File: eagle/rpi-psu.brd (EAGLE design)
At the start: 50.8 x 50.8 mm, 19 parts, among them IC1 LD117AV33, IC2 TINY85P, Q1 TIP125, T1 2N2222

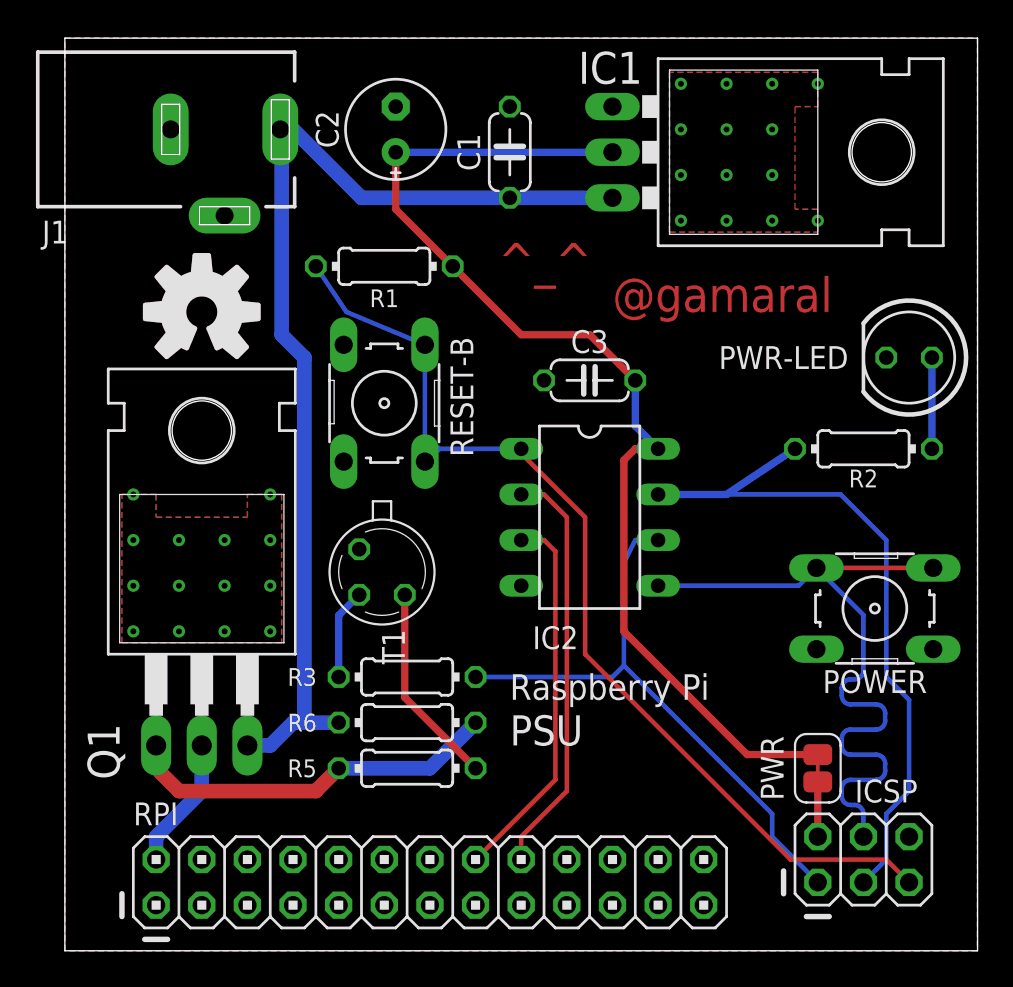
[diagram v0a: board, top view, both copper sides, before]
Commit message: Updated to R3.
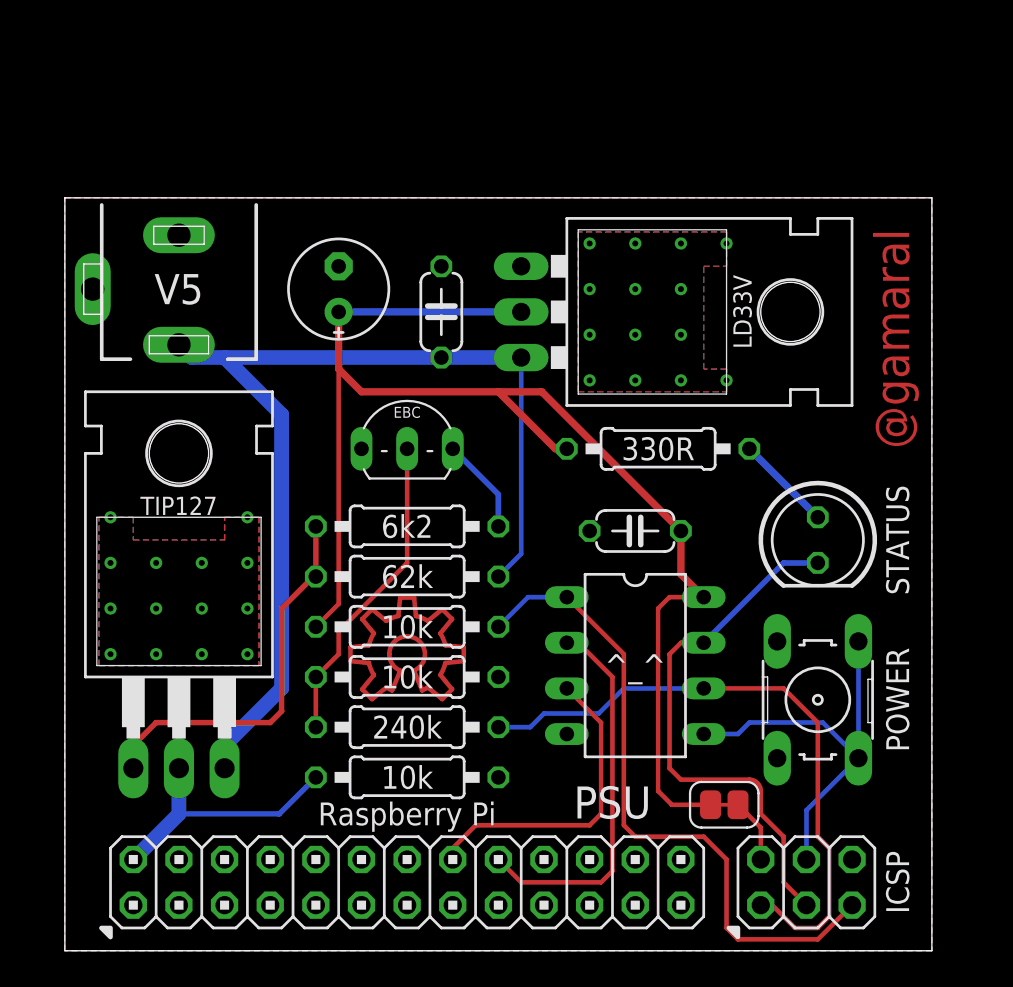
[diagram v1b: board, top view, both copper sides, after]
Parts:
- removed POWER: PWR, switch-omron:B3F-10XX
- removed PWR: (no value), gamaral:SJ-BRIDGED
- removed PWR-LED: STATUS, led:LED5MM
- removed RESET-B: RESET, switch-omron:B3F-10XX
- added R4, R7: 10k, resistor:0207/10
- added SJ1: (no value), gamaral:SJ-BRIDGED
- added STATUS-LED: (no value), led:LED5MM
- added SW1: (no value), switch-omron:B3F-10XX
- R1, R2, R3, R5, R6: device resistor:0204/7 -> resistor:0207/10
- T1: value 2N2222 -> 2N2222A; device transistor:TO18 -> transistor:TO92-EBC
- moved R1 20.1 mm to (19.1, 18.0), turned to 0 degrees
- moved R5 13.5 mm to (19.1, 23.6)
- moved R2 11.4 mm to (33.0, 27.9)
- moved IC1 10.2 mm to (29.2, 35.6)
- moved C1 9.67 mm to (21.0, 35.6)
- moved C2 9.44 mm to (15.2, 36.8)
- moved J1 9.25 mm to (6.35, 36.8), turned to 180 degrees
- moved C3 8.76 mm to (31.8, 23.4)
- moved IC2 8.64 mm to (31.8, 15.9)
- moved T1 8.25 mm to (19.1, 29.2), turned to 0 degrees
- moved R6 8.13 mm to (19.1, 20.8), turned to 0 degrees
- moved ICSP 3.42 mm to (41.3, 3.81)
- moved R3 2.79 mm to (19.1, 12.4)
- moved Q1 1.80 mm to (6.35, 16.5)
- moved RPI 1.27 mm to (19.1, 3.81)
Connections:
- net +3V3: now also R2.1, SJ1.2; no longer PWR.2
- net GND: now also R4.1, R7.1, SW1.1, SW1.2, T1.E; no longer POWER.1, POWER.2, PWR-LED.K, RESET-B.3, RESET-B.4, T1.1
- net ICSP-VCC: now also SJ1.1; no longer PWR.1
- net N$1: now also STATUS-LED.A; no longer PWR-LED.A
- net N$3: now also R7.2
- net N$5: now also R4.2, T1.B; no longer T1.2
- net N$6: now also T1.C; no longer T1.3
- net RESET: no longer RESET-B.1, RESET-B.2
- net RPI-LED: now also STATUS-LED.K; no longer R2.1
- net RPI-USR: now also SW1.3, SW1.4; no longer POWER.3, POWER.4
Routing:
- net RESET: track 56.1 -> 36.9 mm
- net RPI-USR: track 40.4 -> 23.0 mm
- net +3V3: track 62.2 -> 76.5 mm
- net N$5: track 5.05 -> 17.6 mm
- net RPI-LED: track 39.0 -> 29.7 mm
- net N$3: track 7.40 -> 14.6 mm
- net N$6: track 11.3 -> 5.37 mm
- net RPI-OUT: track 21.2 -> 17.5 mm
- net RPI-IN: track 23.2 -> 21.3 mm
- net +5V: track 59.2 -> 57.6 mm
- net RPI-PWR: track 33.5 -> 35.1 mm
- net ICSP-VCC: track 3.05 -> 3.57 mm
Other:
- board size 50.8 x 50.8 mm -> 48.3 x 41.9 mm
- board text added: "EBC"
- board text added: "LD33V"
- board text added: "POWER"
- board text added: "STATUS"
- board text added: "TIP127"
- board text added: "V5"
